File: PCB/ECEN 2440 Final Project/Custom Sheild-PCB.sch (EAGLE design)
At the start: 14 parts

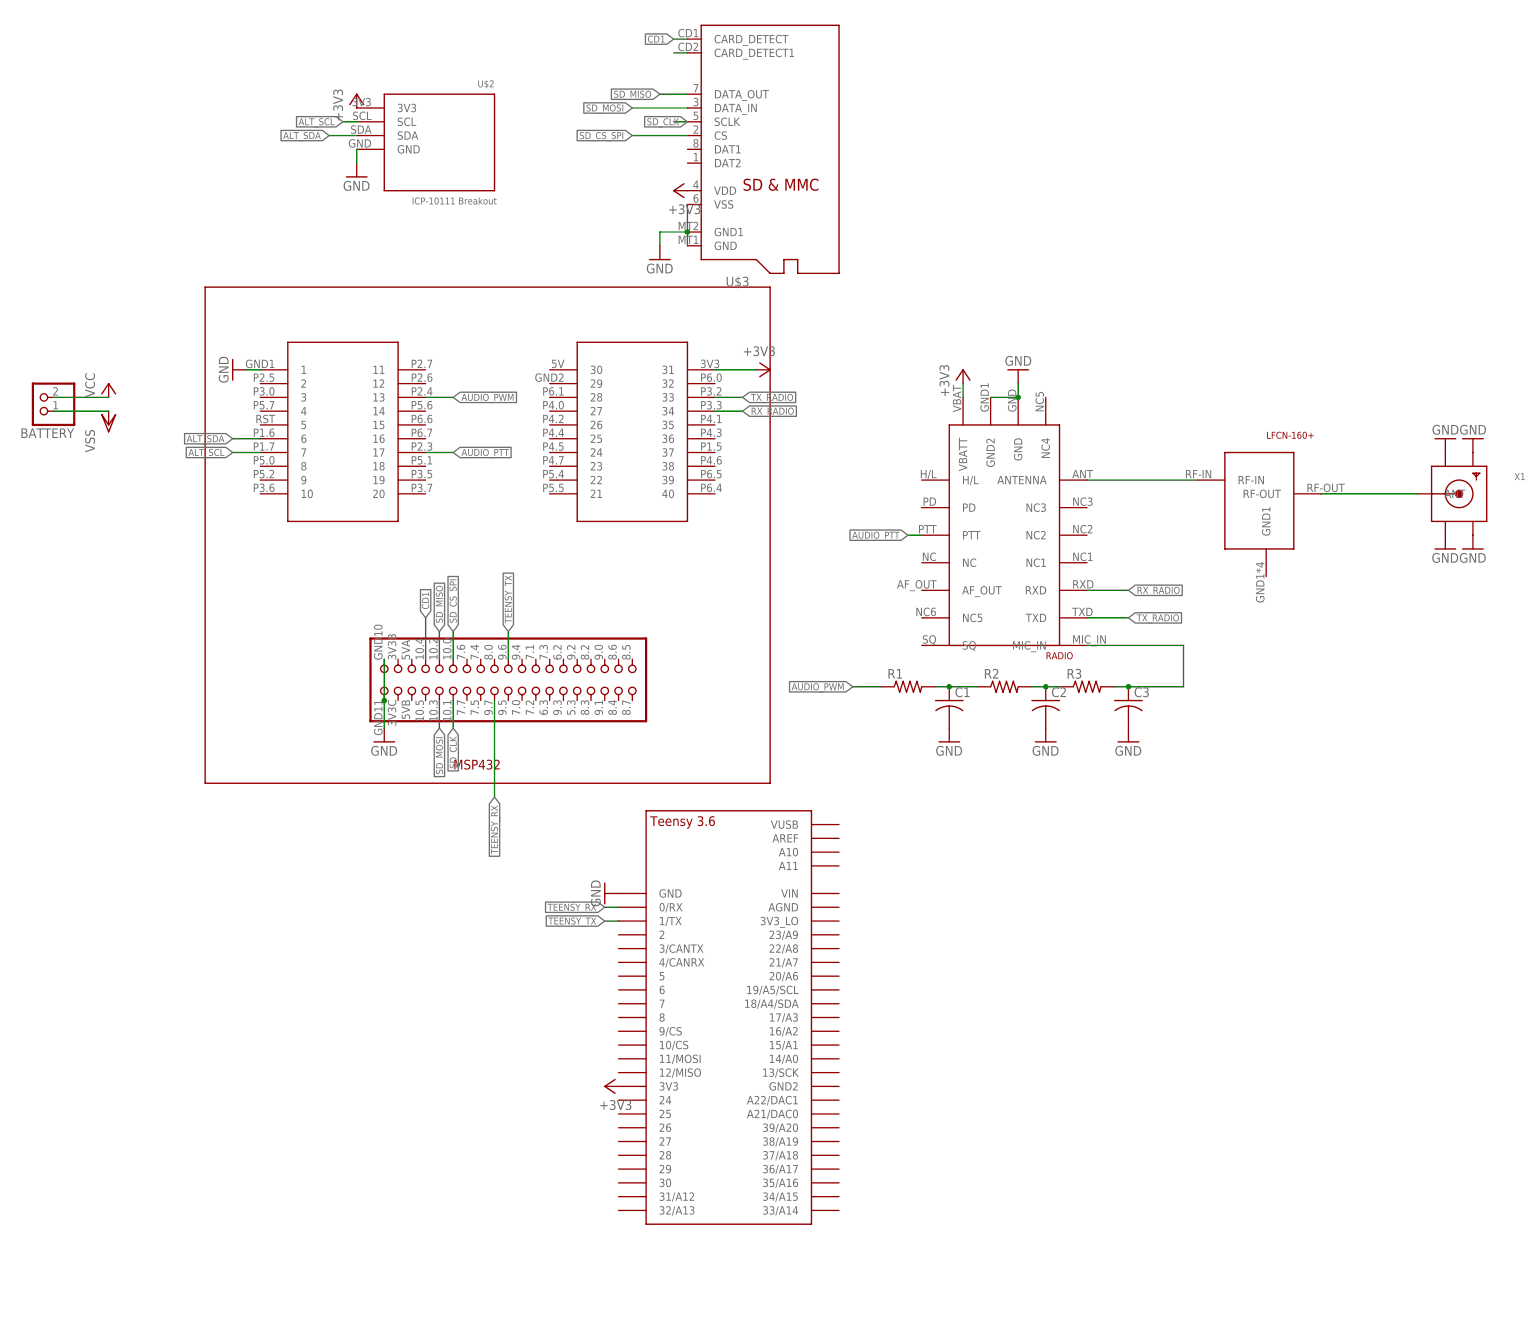
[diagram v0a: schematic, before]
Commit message: PDR schematic and board
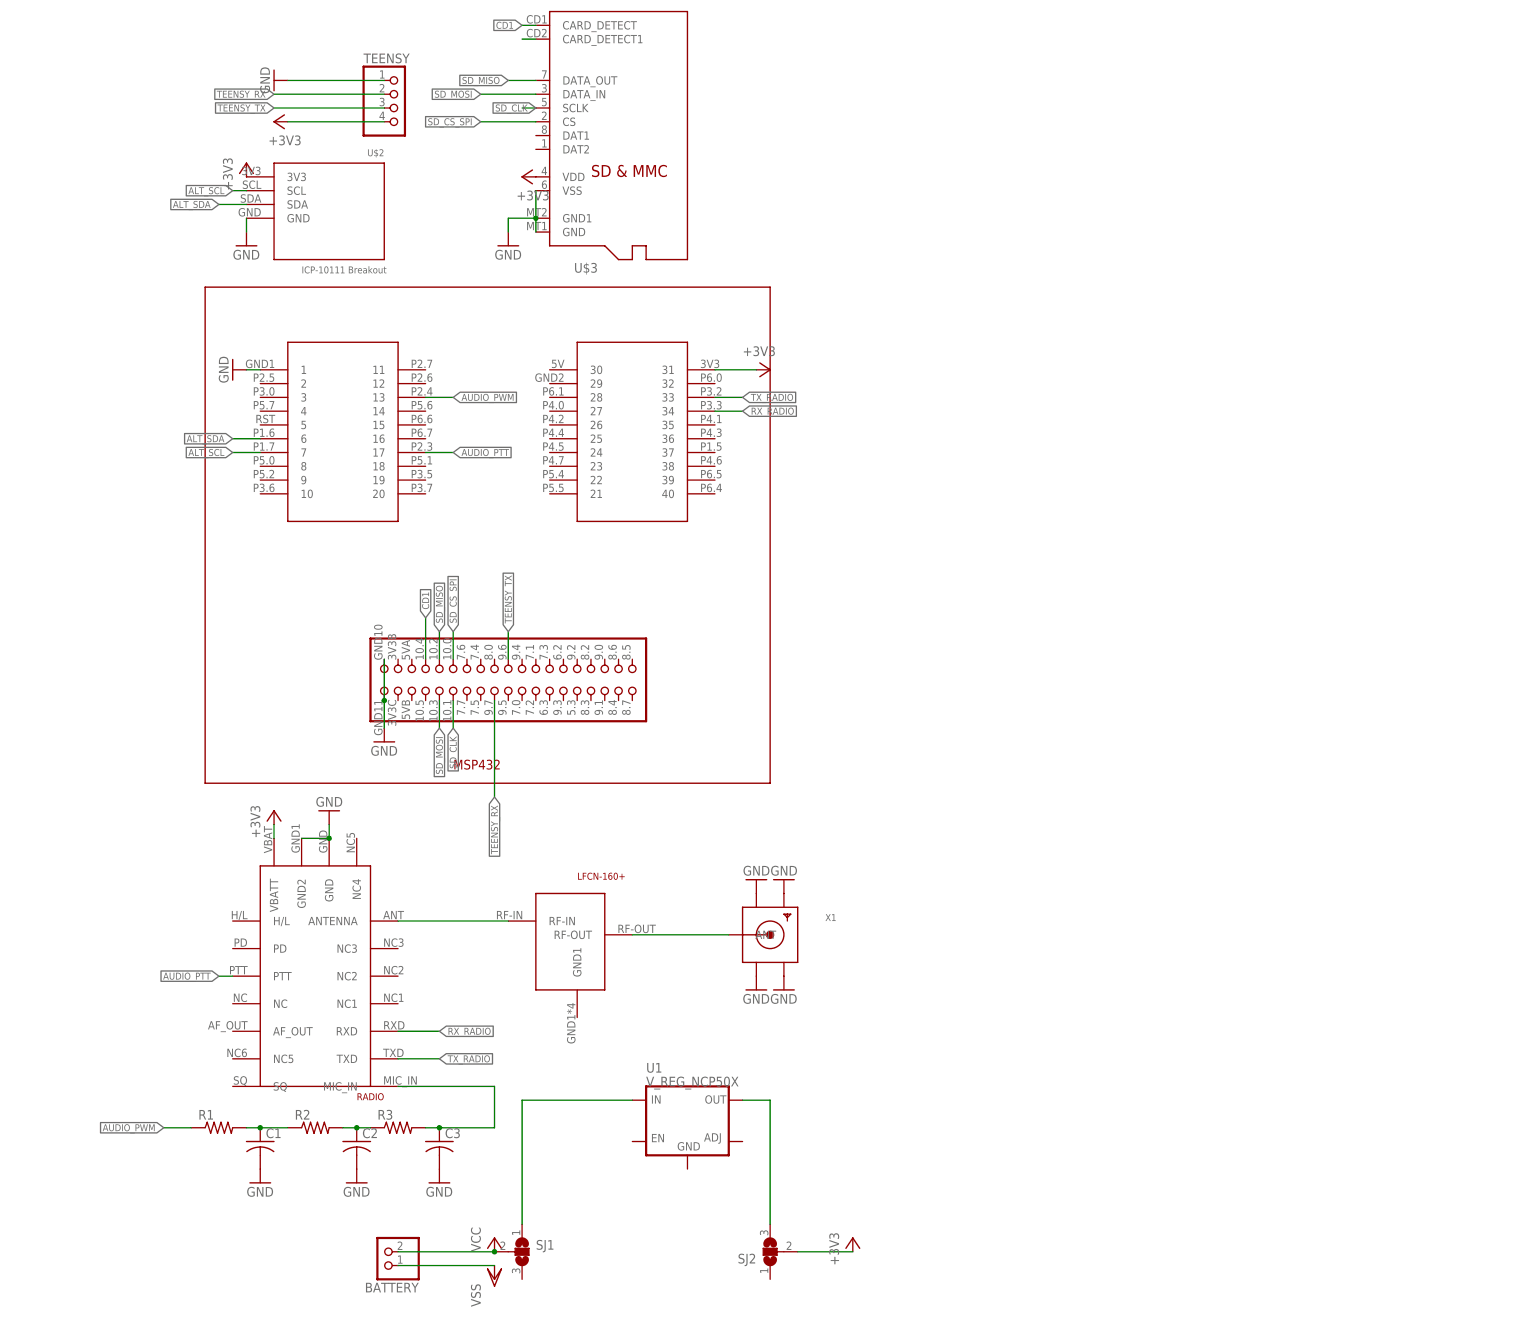
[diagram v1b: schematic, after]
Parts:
- removed U$5: TEENSY_3.5/3.6_BASIC, Teensy356:TEENSY_3.5/3.6_BASIC
- added SJ1, SJ2: (no value), jumper:SJ2WW
- added TEENSY: (no value), pinhead:PINHD-1X4
- added U1: V_REG_NCP50X, SparkFun-IC-Power:V_REG_NCP50X
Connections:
- new net N$7: SJ1.1, U1.IN
- new net N$8: SJ2.3, U1.OUT
- net +3V3: now also SJ2.2, TEENSY.4; no longer U$5.3V3
- net GND: now also TEENSY.1; no longer U$5.GND
- net TEENSY_RX: now also TEENSY.2; no longer U$5.0/RX
- net TEENSY_TX: now also TEENSY.3; no longer U$5.1/TX
- net VCC: now also SJ1.2
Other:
- moved on the sheet: BATTERY, C1, C2, C3, R1, R2, R3, U$2, X1
